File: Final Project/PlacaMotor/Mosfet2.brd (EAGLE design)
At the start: 36.3 x 37.5 mm, 14 parts, among them IC1 ATTINY44-SSU

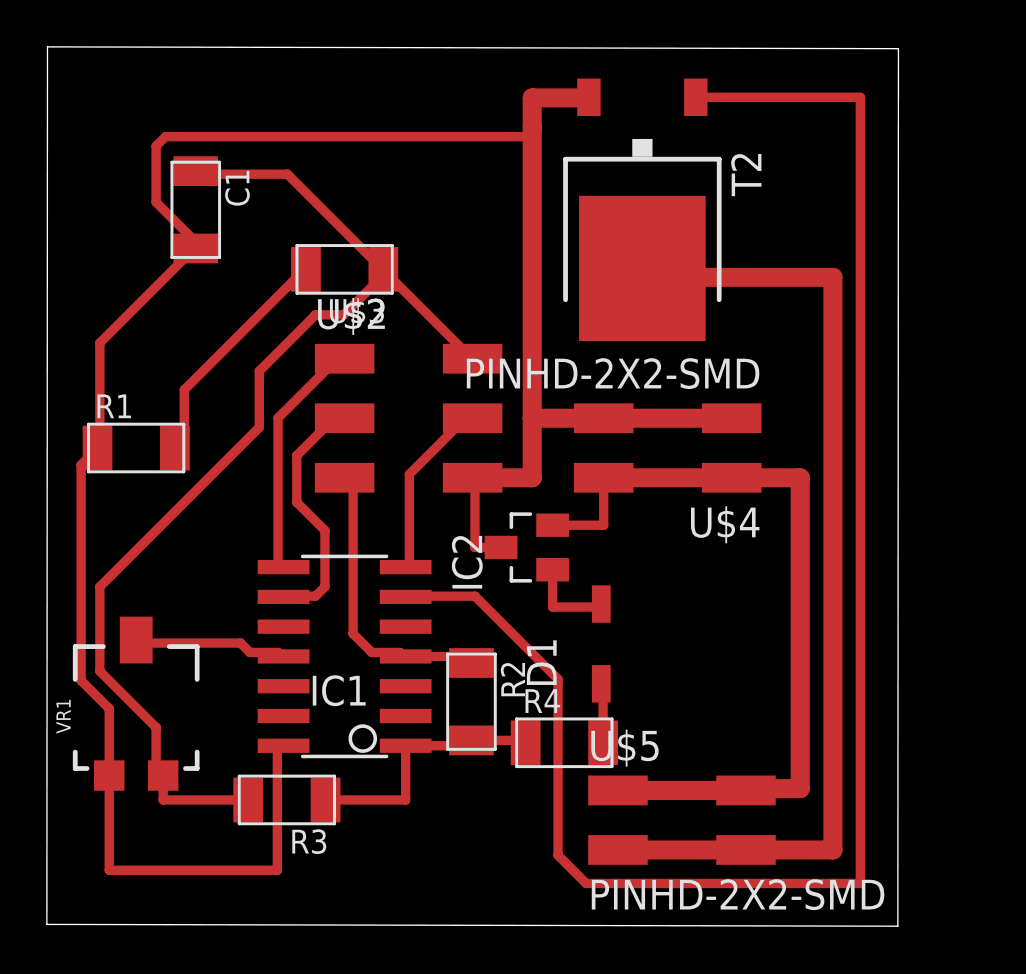
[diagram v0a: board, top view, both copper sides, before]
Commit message: Placa FTDI
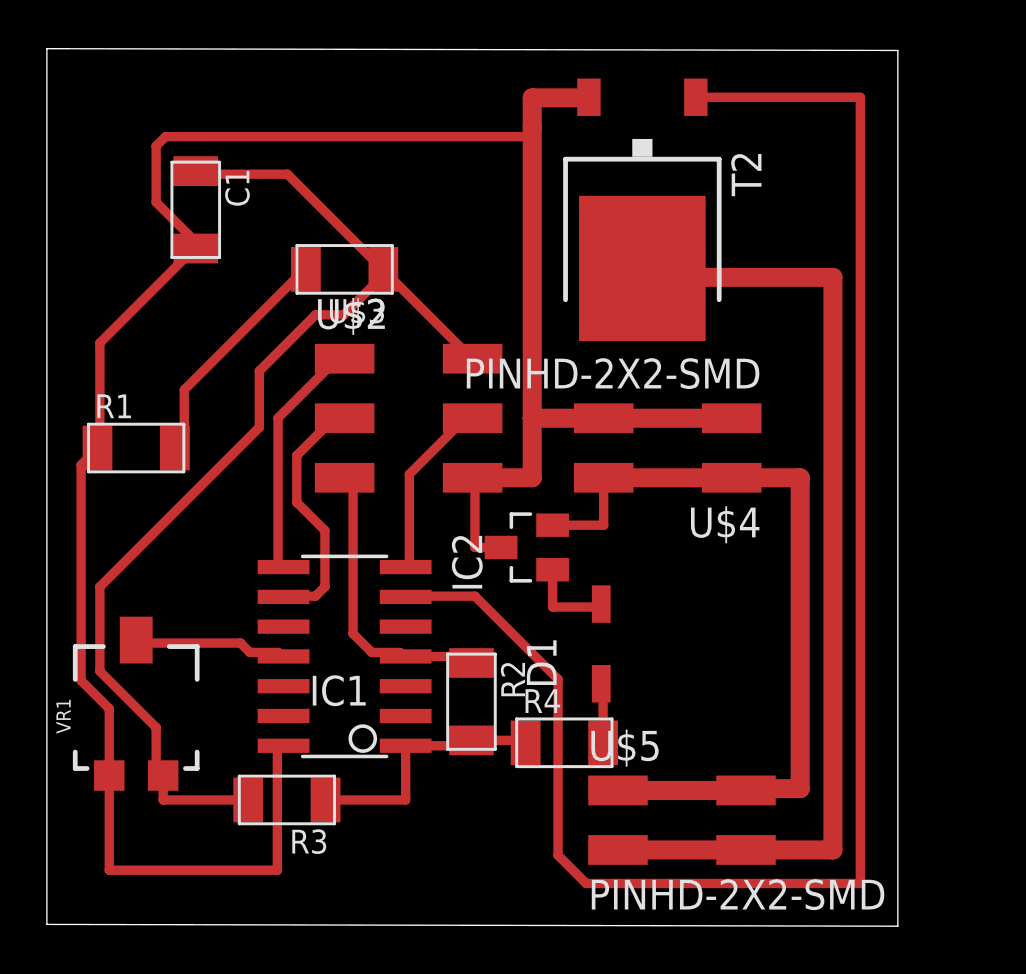
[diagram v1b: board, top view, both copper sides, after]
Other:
- board size 36.3 x 37.5 mm -> 36.3 x 37.4 mm
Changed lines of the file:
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@@
 <plain>
 <wire x1="0" y1="0" x2="36.2968" y2="-0.0762" width="0" layer="20"/>
-<wire x1="36.2968" y1="-0.0762" x2="36.3222" y2="37.3534" width="0" layer="20"/>
-<wire x1="36.3222" y1="37.3534" x2="0.0254" y2="37.4296" width="0" layer="20"/>
-<wire x1="0.0254" y1="37.4296" x2="0" y2="0" width="0" layer="20"/>
+<wire x1="36.2968" y1="-0.0762" x2="36.2968" y2="37.2772" width="0" layer="20"/>
+<wire x1="36.2968" y1="37.2772" x2="0" y2="37.3534" width="0" layer="20"/>
+<wire x1="0" y1="37.3534" x2="0" y2="0" width="0" layer="20"/>
 </plain>
 <attributes>
